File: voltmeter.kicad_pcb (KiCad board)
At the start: 2 copper layers, 96.5 x 26.9 mm, 34 parts, among them CON1 AVR-ISP-6, J1 Conn_01x02, J2 Conn_01x02, J3 Conn_01x01, J4 Conn_01x01, J5 Conn_01x01, J6 Conn_01x01, J7 Conn_01x01, J8 Conn_01x01, J9 Conn_01x01, Q1 BC547, Q2 BC547, Q3 BC547, Q4 BC547, U1 AZ1117-3.3, U2 ATMEGA328P-AU, U3 7SEGMENT_CC, U4 7SEGMENT_CC, U5 7SEGMENT_CC, U6 7SEGMENT_CC, Y1 Crystal

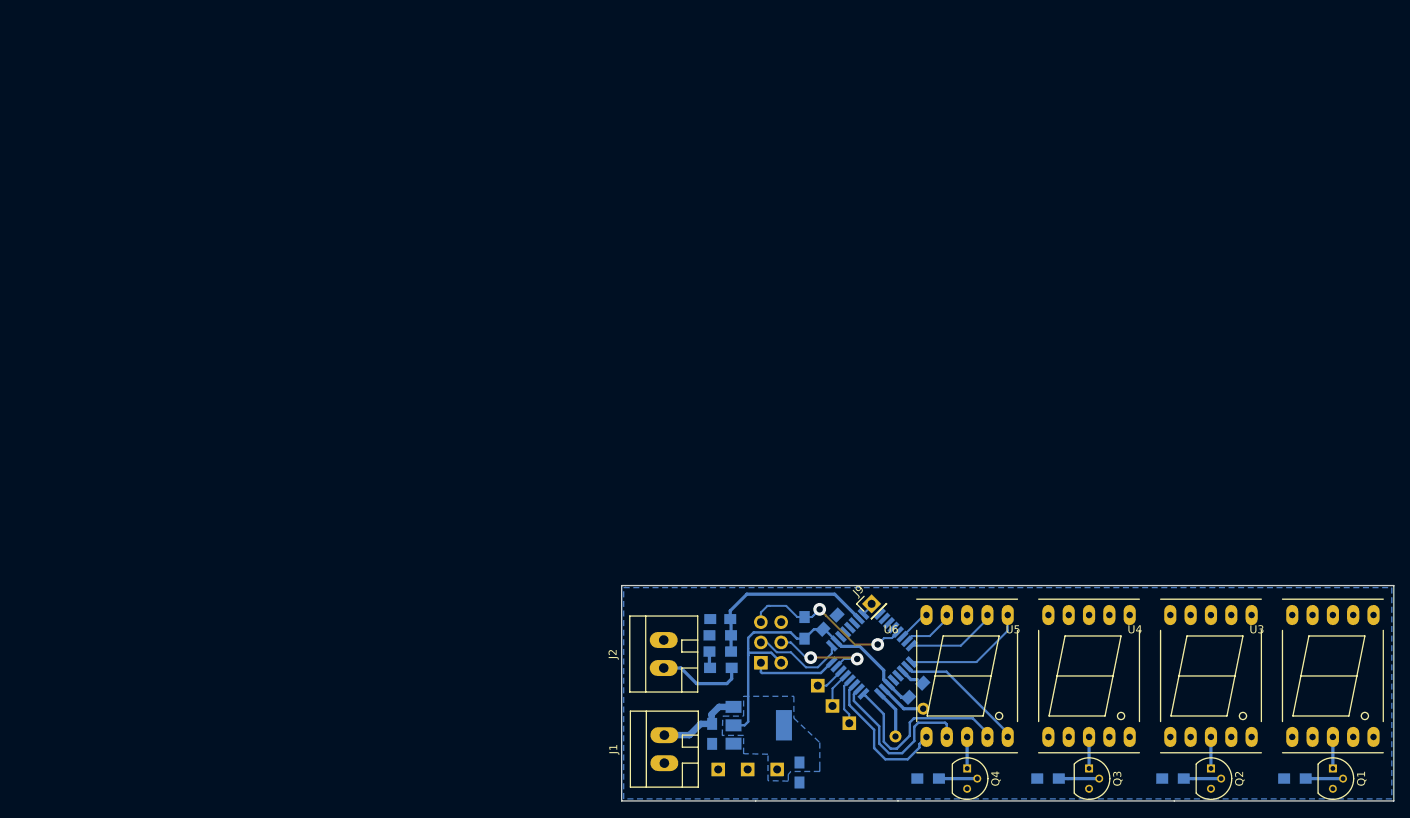
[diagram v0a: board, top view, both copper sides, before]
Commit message: Update PCB
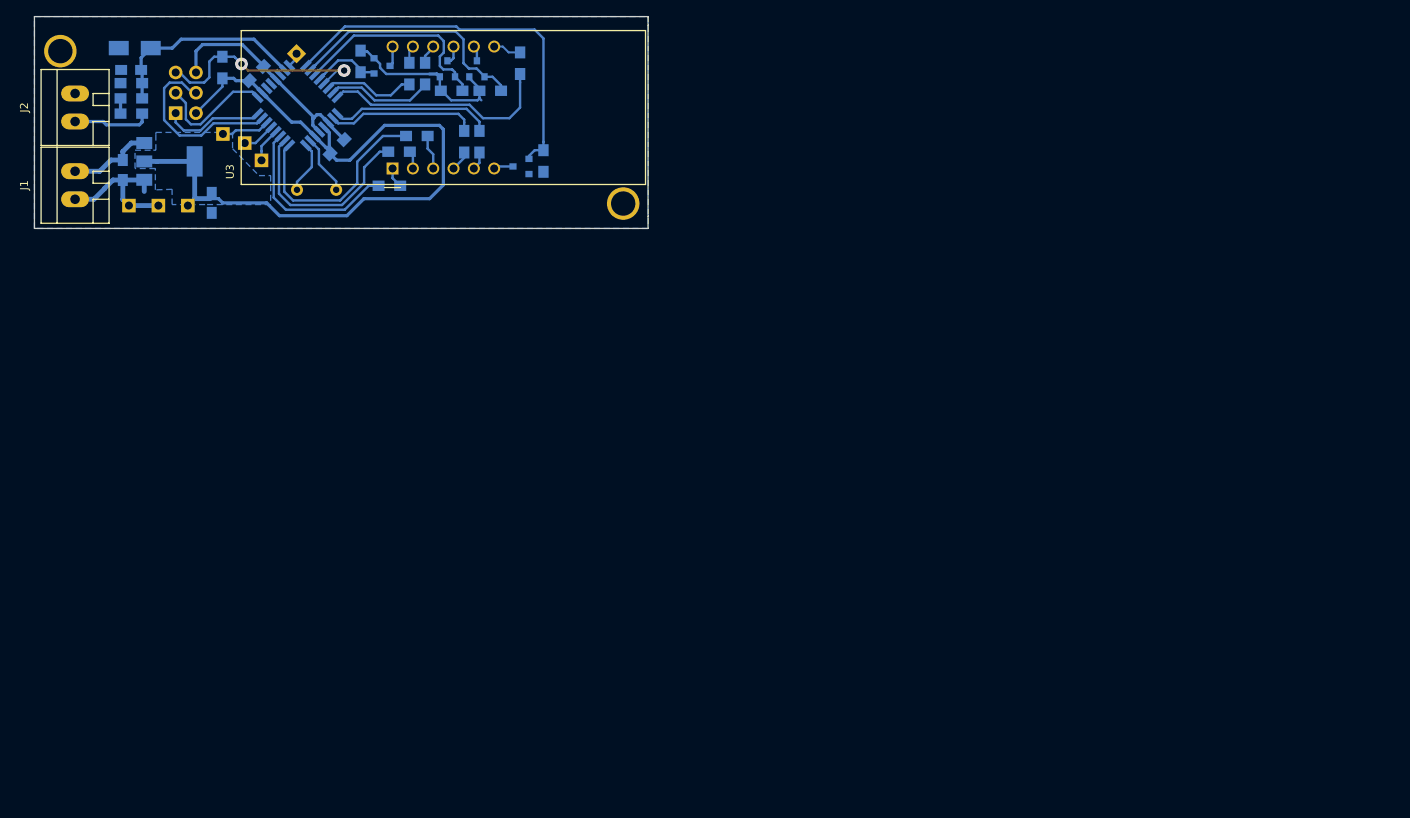
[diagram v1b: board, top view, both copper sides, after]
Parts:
- removed U4, U5, U6: 7SEGMENT_CC, Displays_7-Segment:7SegmentLED_LTS6760_LTS6780
- added D1: 3v6, Diodes_SMD:D_SMA, B.Cu at (30.6, 26.3)
- added R10: 100, Resistors_SMD:R_0805_HandSoldering, B.Cu at (71.8, 38.0)
- added R11: 100, Resistors_SMD:R_0805_HandSoldering, B.Cu at (65.8, 37.3)
- added R12: 100, Resistors_SMD:R_0805_HandSoldering, B.Cu at (63.6, 39.2)
- added R13: 100, Resistors_SMD:R_0805_HandSoldering, B.Cu at (62.4, 43.5)
- added R14: 4K7, Resistors_SMD:R_0805_HandSoldering, B.Cu at (75.0, 31.6)
- added R15: 4K7, Resistors_SMD:R_0805_HandSoldering, B.Cu at (70.2, 31.6)
- added R16: 4K7, Resistors_SMD:R_0805_HandSoldering, B.Cu at (58.8, 28.0)
- added R9: 100, Resistors_SMD:R_0805_HandSoldering, B.Cu at (73.7, 38.0)
- added REF**: 1pin, Connectors:1pin, B.Cu at (21.3, 26.7)
- added REF**: 1pin, Connectors:1pin, B.Cu at (91.6, 45.7)
- C1: value C -> 1U
- C2: value C -> 1u
- C3, C4, C5: value C -> 0.1u
- J9: moved to B.Cu
- Q1, Q2, Q3, Q4: value BC547 -> 2N7002; footprint TO_SOT_Packages_THT:TO-92_Molded_Narrow -> TO_SOT_Packages_SMD:SOT-23; moved to B.Cu
- R1: value R -> 10K
- R2: value R -> 4K7
- R3: value 1kR -> 1K
- R4, R7, R8: value R -> 100
- R5: value R -> 2K2
- R6: value R -> 22K
- U3: value 7SEGMENT_CC -> CA56-12EWA; footprint Displays_7-Segment:7SegmentLED_LTS6760_LTS6780 -> Displays_7-Segment:CA56-12EWA
- Y1: value Crystal -> 16M
- moved U3 133.6 mm to (62.8, 41.3), turned to 90 degrees
- moved R4 129.9 mm to (64.9, 29.5), turned to 270 degrees
- moved Q2 126.8 mm to (73.3, 28.9), turned to 90 degrees
- moved Q1 126.3 mm to (78.9, 41.1), turned to 180 degrees
- moved R2 121.6 mm to (81.7, 40.4), turned to 270 degrees
- moved Q3 118.7 mm to (69.7, 28.9), turned to 90 degrees
- moved R7 117.6 mm to (66.9, 29.5), turned to 270 degrees
- moved Q4 114.3 mm to (61.5, 28.5), turned to 0 degrees
- moved R8 102.9 mm to (78.7, 28.2), turned to 270 degrees
- moved C3 102.3 mm to (40.2, 45.6)
- moved J3 102.0 mm to (33.5, 46.0)
- moved J4 102.0 mm to (29.8, 46.0)
- moved J5 102.0 mm to (37.2, 46.0)
- moved J1 102.0 mm to (23.1, 43.4)
- moved U1 102.0 mm to (34.9, 40.5)
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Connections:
- Q1 pad 2: Net-(Q1-Pad2) -> GND
- Q1 pad 3: GND -> Net-(Q1-Pad3)
- Q2 pad 2: Net-(Q2-Pad2) -> GND
- Q2 pad 3: GND -> Net-(Q2-Pad3)
- Q3 pad 2: Net-(Q3-Pad2) -> GND
- Q3 pad 3: GND -> Net-(Q3-Pad3)
- Q4 pad 2: Net-(Q4-Pad2) -> GND
- Q4 pad 3: GND -> Net-(Q4-Pad3)
- R2 pad 1: Net-(Q1-Pad2) -> Net-(Q1-Pad1)
- R2 pad 2: Net-(R2-Pad2) -> GND
- R4 pad 1: Net-(Q2-Pad2) -> Net-(R4-Pad1)
- R7 pad 1: Net-(Q3-Pad2) -> Net-(R7-Pad1)
- R8 pad 1: Net-(Q4-Pad2) -> Net-(R8-Pad1)
- U2 pad 1: Net-(U2-Pad1) -> Net-(R9-Pad2)
- U2 pad 10: Net-(U2-Pad10) -> Net-(R12-Pad2)
- U2 pad 11: Net-(U2-Pad11) -> Net-(R13-Pad2)
- U2 pad 2: Net-(U2-Pad2) -> Net-(R10-Pad2)
- U2 pad 25: Net-(R2-Pad2) -> Net-(Q1-Pad1)
- U2 pad 26: Net-(R4-Pad2) -> Net-(Q2-Pad1)
- U2 pad 27: Net-(R7-Pad2) -> Net-(Q3-Pad1)
- U2 pad 28: Net-(R8-Pad2) -> Net-(Q4-Pad1)
- U2 pad 30: Net-(U2-Pad30) -> Net-(R4-Pad2)
- U2 pad 31: Net-(U2-Pad31) -> Net-(R7-Pad2)
- U2 pad 32: Net-(U2-Pad32) -> Net-(R8-Pad2)
- U2 pad 9: Net-(U2-Pad9) -> Net-(R11-Pad2)
- U3 pad 1: Net-(U2-Pad11) -> Net-(R13-Pad1)
- U3 pad 10: Net-(U2-Pad30) -> Net-(R7-Pad1)
- U3 pad 2: Net-(U2-Pad10) -> Net-(R12-Pad1)
- U3 pad 3: Net-(Q1-Pad1) -> Net-(R11-Pad1)
- U3 pad 4: Net-(U2-Pad9) -> Net-(R10-Pad1)
- U3 pad 5: Net-(U2-Pad2) -> Net-(R9-Pad1)
- U3 pad 6: Net-(U2-Pad1) -> Net-(Q1-Pad3)
- U3 pad 7: Net-(U2-Pad32) -> Net-(R8-Pad1)
- U3 pad 8: Net-(Q1-Pad1) -> Net-(Q2-Pad3)
- U3 pad 9: Net-(U2-Pad31) -> Net-(Q3-Pad3)
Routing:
- net GND: track 2.28 -> 70.2 mm
- net +3V3: track 42.9 -> 95.7 mm
- net Net-(Q1-Pad1): track 3.94 -> 48.8 mm
- net Net-(R8-Pad2): track 0.00 -> 29.2 mm
- net Net-(Q2-Pad1): track 3.94 -> 31.1 mm
- net Net-(R11-Pad2): track 0.00 -> 26.6 mm
- net Net-(R12-Pad2): track 0.00 -> 25.0 mm
- net Net-(U2-Pad9): track 24.2 -> 0.00 mm
- net Net-(R13-Pad2): track 0.00 -> 23.0 mm
- net Net-(Q3-Pad1): track 3.94 -> 26.7 mm
- net Net-(U2-Pad10): track 21.6 -> 0.00 mm
- net Net-(R9-Pad2): track 0.00 -> 20.4 mm
- net Net-(R10-Pad2): track 0.00 -> 18.9 mm
- net Net-(U2-Pad11): track 18.0 -> 0.00 mm
- net Net-(U2-Pad2): track 16.5 -> 0.00 mm
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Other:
- board size 96.5 x 26.9 mm -> 76.7 x 26.5 mm
- net class Default: clearance 0.254 -> 0.2032
- rule trace_clearance: 0.254 -> 0.2032
